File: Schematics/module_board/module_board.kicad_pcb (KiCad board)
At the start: 2 copper layers, 30 x 30 mm, 35 parts, among them J1 Conn_01x01_Male, J11 Conn_01x01_Male, J12 Conn_01x01_Male, J13 Conn_01x01_Male, J14 Conn_01x01_Male, J15 Conn_01x01_Male, J16 Conn_01x01_Male, J17 Conn_01x01_Male, J2 Conn_01x01_Male, J3 Conn_01x01_Male, J4 Conn_01x01_Male, J5 Conn_01x06_Male, U1 RP2040, U2 W25Q16JVSSIQ, Y1 ABLS-12.000MHZ-B4-T

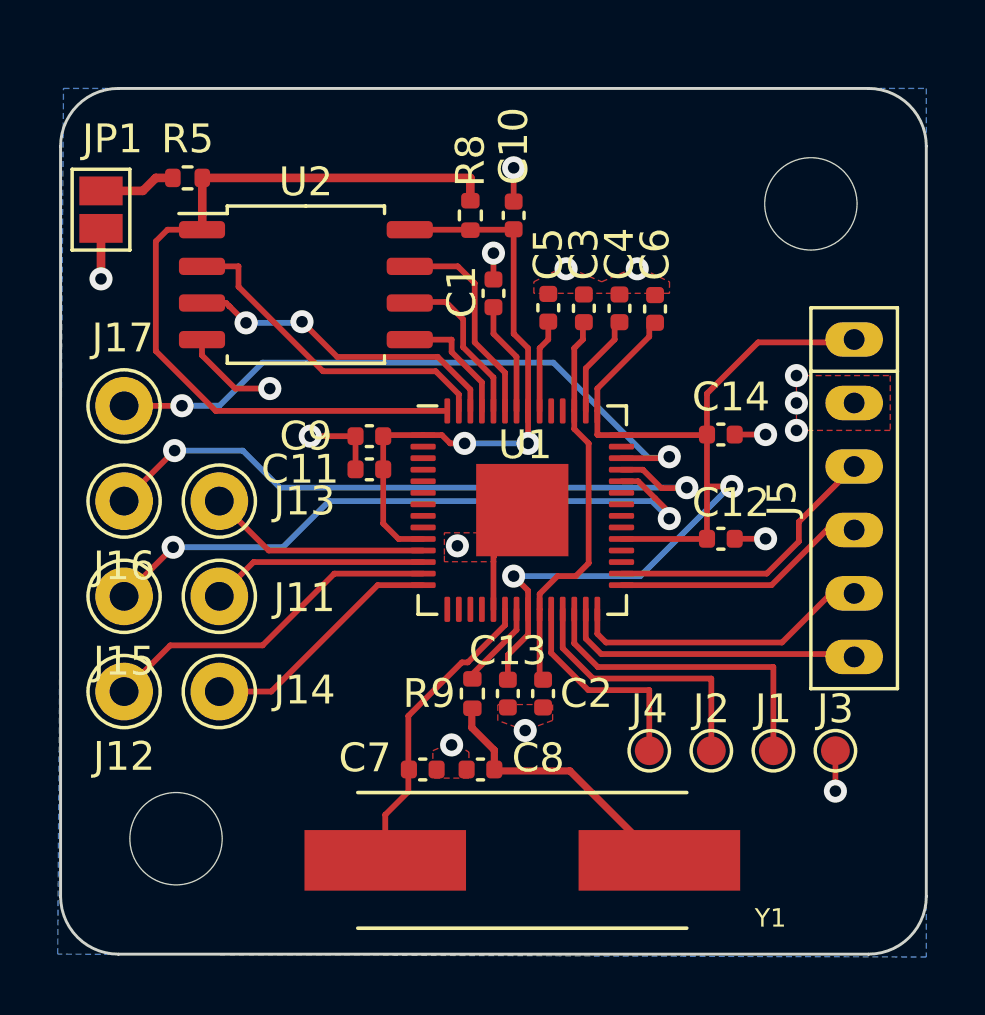
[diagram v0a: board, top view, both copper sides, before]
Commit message: Module updates
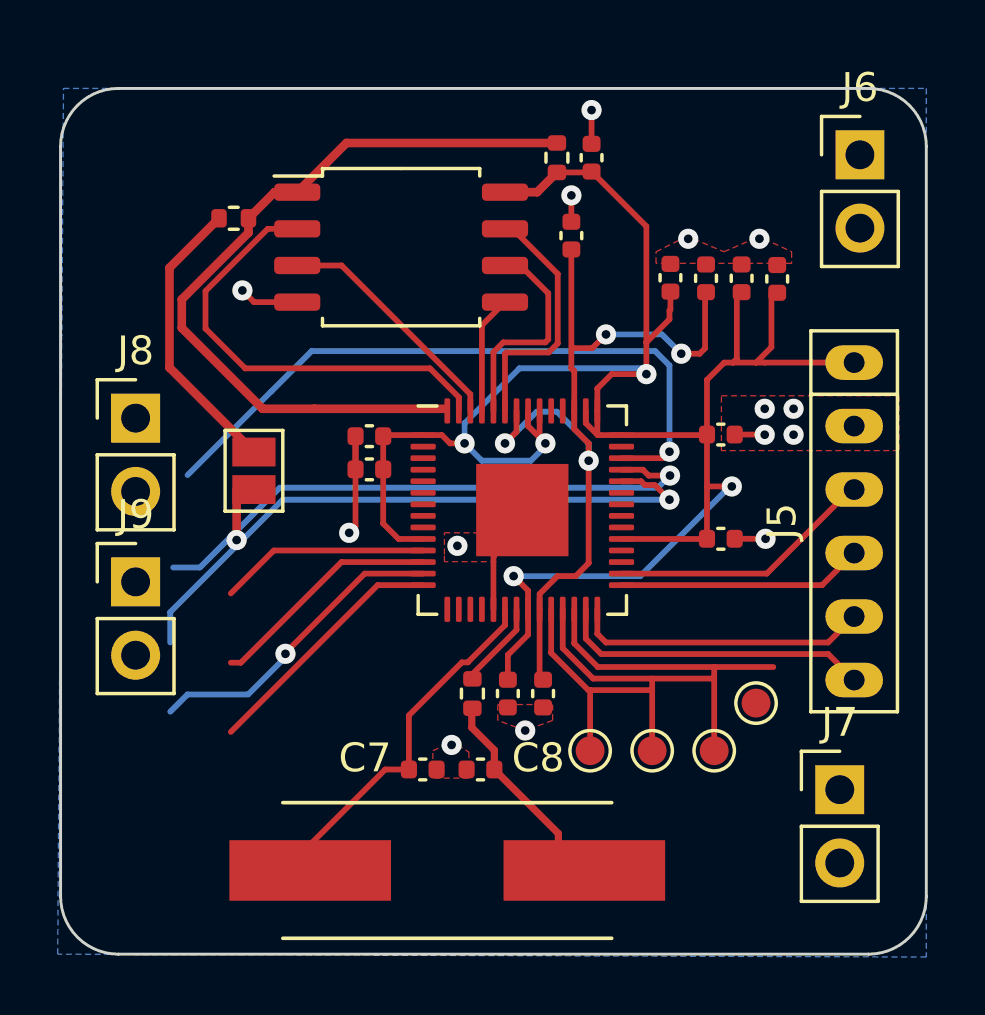
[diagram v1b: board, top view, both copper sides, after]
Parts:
- removed J11, J12, J13, J14, J15, J16, J17: Conn_01x01_Male, Connector_Pin:Pin_D1.0mm_L10.0mm
- removed REF**, hello: MountingHole_3.2mm_M3, MountingHole:MountingHole_3.2mm_M3
- added J6: Conn_01x02_Female, Connector_PinHeader_2.54mm:PinHeader_1x02_P2.54mm_Vertical, F.Cu at (172.7, 77.3)
- added J7: Conn_01x02_Female, Connector_PinHeader_2.54mm:PinHeader_1x02_P2.54mm_Vertical, F.Cu at (172.0, 99.3)
- added J8: Conn_01x02_Female, Connector_PinHeader_2.54mm:PinHeader_1x02_P2.54mm_Vertical, F.Cu at (147.6, 86.4)
- added J9: Conn_01x02_Female, Connector_PinHeader_2.54mm:PinHeader_1x02_P2.54mm_Vertical, F.Cu at (147.6, 92.1)
- J5: footprint Prototroller:Mag_Pogo_6P_P2.2mm_Male -> prototroller_footprints:Mag_Pogo_6P_P2.2mm_Male
- Y1: footprint ABLS-12:XTAL_ABLS-12.000MHZ-B4-T -> prototroller_footprints:XTAL_ABLS-12.000MHZ-B4-T
- moved JP1 10.5 mm to (151.7, 88.2)
- moved C3 4.36 mm to (167.4, 81.6)
- moved C6 4.36 mm to (169.8, 81.6)
- moved C4 4.36 mm to (168.6, 81.6)
- moved C5 4.36 mm to (166.1, 81.6)
- moved R8 3.61 mm to (162.2, 77.4)
- moved U2 3.55 mm to (156.8, 80.5)
- moved C10 3.36 mm to (163.4, 77.4)
- moved C1 3.36 mm to (162.7, 80.1)
- moved J3 3.21 mm to (169.1, 96.3)
- moved Y1 2.62 mm to (158.4, 102.1)
- moved R5 2.13 mm to (151.0, 79.5)
- moved J2 2.05 mm to (165.5, 98.0)
- moved J4 2.05 mm to (163.3, 98.0)
- moved J1 2.05 mm to (167.7, 98.0)
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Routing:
- net +3V3: track 62.9 -> 75.5 mm, vias 4 -> 5
- net +1V1: track 17.8 -> 29.0 mm, vias 0 -> 4
- net /BOOTSEL_N: track 2.68 -> 10.0 mm
- net /QSPI_SD1: track 11.7 -> 15.6 mm
- net /GPIO27_ADC1: track 23.3 -> 20.3 mm, vias 2 -> 1
- net /QSPI_SD2: track 11.3 -> 8.42 mm, vias 2 -> 0
- net Net-(C8-Pad2): track 9.48 -> 6.87 mm
- net /QSPI_SCLK: track 5.72 -> 7.62 mm
- net /XTAL_IN: track 10.8 -> 12.7 mm
- net /QSPI_NSS: track 28.3 -> 26.5 mm
- net /QSPI_SD3: track 7.35 -> 8.84 mm
- net /SPI1_SCK: track 12.1 -> 10.8 mm, vias 0 -> 1
- net /RX: track 9.78 -> 10.9 mm
- net /GPIO26_ADC0: track 22.8 -> 21.9 mm, vias 2 -> 1
- net GND: track 17.5 -> 16.6 mm, vias 16 -> 15
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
